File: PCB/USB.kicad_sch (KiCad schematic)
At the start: 17 parts, among them J1 USB4510-03-1-A_REVA, J1101 USB4510-03-1-A_REVA, U1101 HSP051-4M10, U2 HSP051-4M10

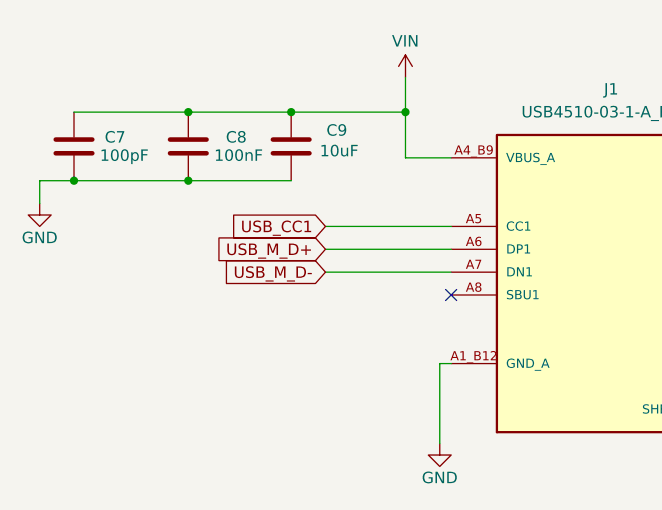
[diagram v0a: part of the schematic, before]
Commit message: UPDATE
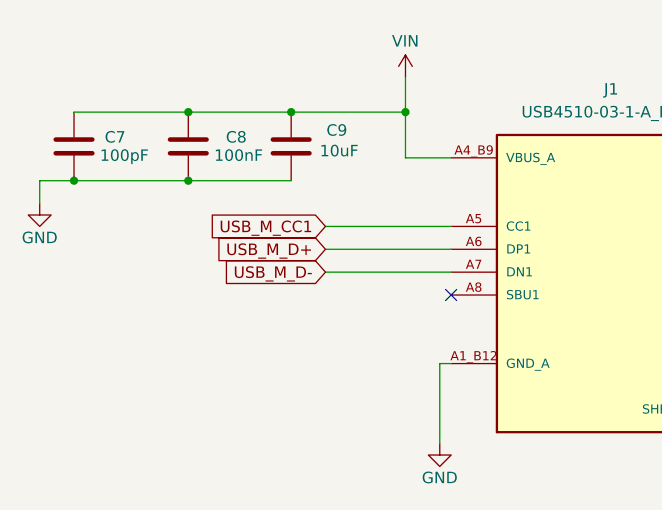
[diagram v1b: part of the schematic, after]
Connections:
- net USB_CC1: no longer J1.A5 (CC1)
- net USB_M_CC1: now also J1.A5 (CC1)
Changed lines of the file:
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@@
 		)
 	)
-	(global_label "USB_CC1"
+	(global_label "USB_M_CC1"
 		(shape input)
 		(at 88.9 118.11 180)
@@
 		)
 		(property "Intersheetrefs" "${INTERSHEET_REFS}"
-			(at 77.3877 118.11 0)
+			(at 74.9687 118.11 0)
 			(effects
 				(font
